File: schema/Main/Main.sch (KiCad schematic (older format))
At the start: 3 parts

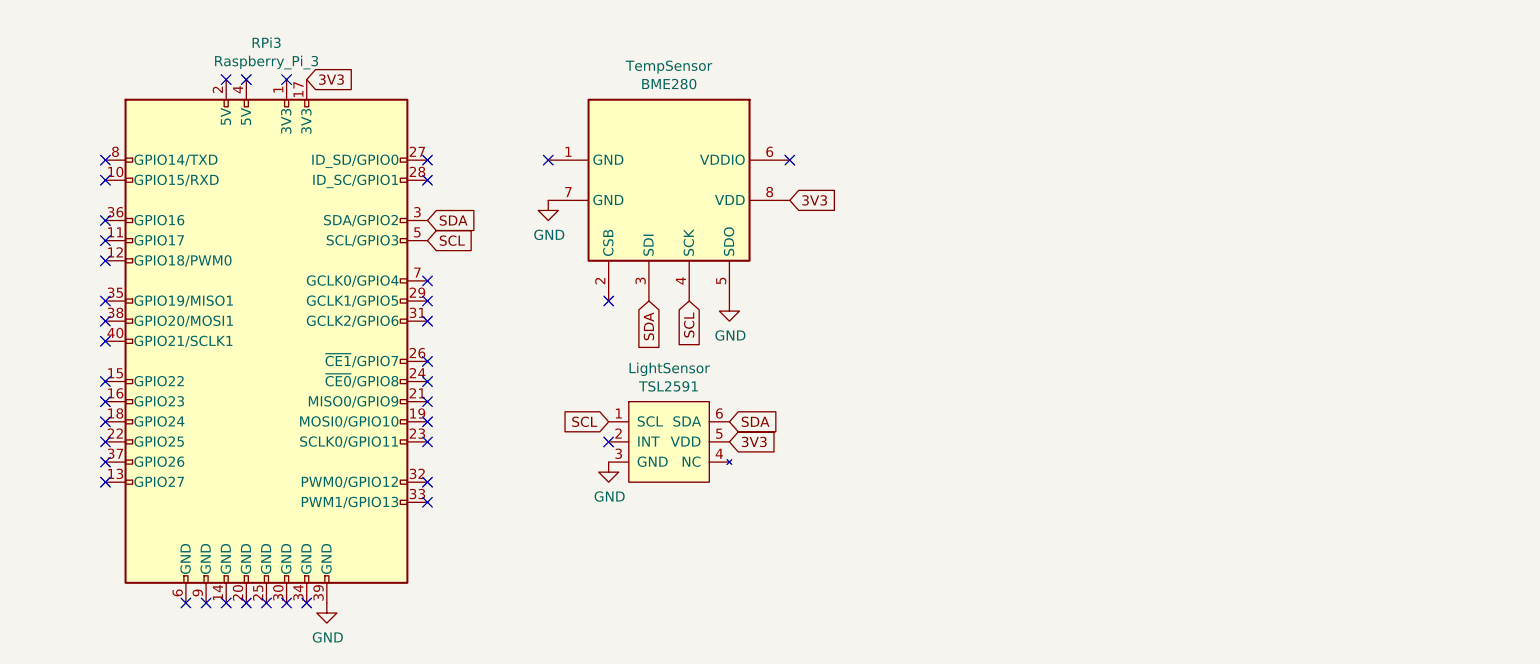
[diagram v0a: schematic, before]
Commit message: update
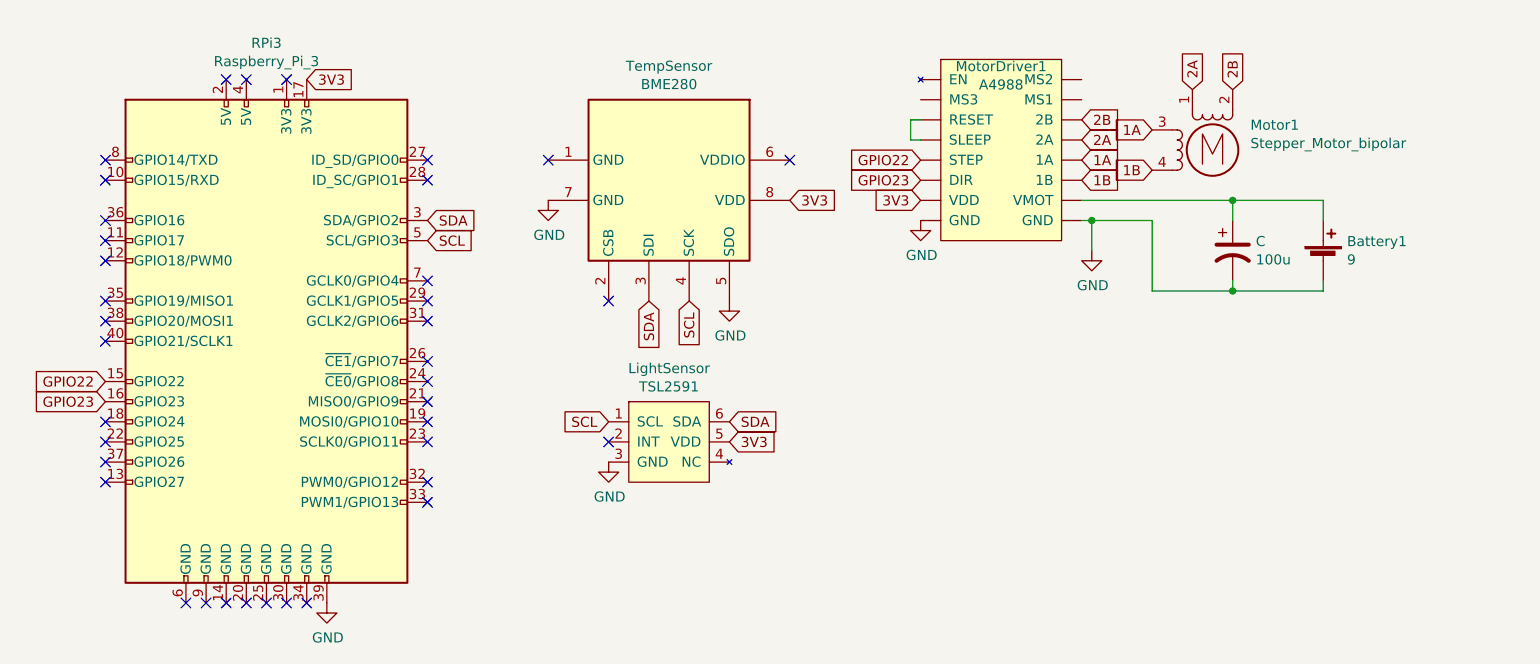
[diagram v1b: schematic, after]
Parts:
- added Battery1: 9, symbol Device:Battery_Cell
- added C: 100u, symbol Device:CP1
- added Motor1: Stepper_Motor_bipolar, symbol Motor:Stepper_Motor_bipolar
- added MotorDriver1: A4988, symbol A4998:A4988
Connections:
- net 3V3: now also MotorDriver1.~ (VMOT)
- net GND: now also Battery1.2 (-), C.2, MotorDriver1.~ (VMOT)
- net GPIO22: now reaches RPi3.15 (GPIO22)
- net GPIO22: now also MotorDriver1.~ (VMOT)
- net GPIO23: now reaches RPi3.16 (GPIO23)
- net GPIO23: now also MotorDriver1.~ (VMOT)
- new net: Battery1.1 (+), C.1, MotorDriver1.~ (VMOT)
- new net 1A: Motor1.3, MotorDriver1.~ (VMOT)
- new net 1B: Motor1.4, MotorDriver1.~ (VMOT)
- new net 2A: Motor1.1, MotorDriver1.~ (VMOT)
- new net 2B: Motor1.2 (-), MotorDriver1.~ (VMOT)
- no-connect marks 40 -> 38
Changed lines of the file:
@@
 NoConn ~ 900  2050
 NoConn ~ 900  2150
-NoConn ~ 900  2350
-NoConn ~ 900  2450
 NoConn ~ 900  2550
 NoConn ~ 900  2650
@@
 $EndComp
 NoConn ~ 3400 2650
+Wire Wire Line
+	4950 1150 4900 1150
+Wire Wire Line
+	4900 1150 4900 1050
+Wire Wire Line
+	4900 1050 4950 1050
+$Comp
+L Motor:Stepper_Motor_bipolar Motor1
+U 1 1 5E3C1483
+P 6400 1200
+F 0 "Motor1" H 6588 1324 50  0000 L CNN
+F 1 "Stepper_Motor_bipolar" H 6588 1233 50  0000 L CNN
+F 2 "" H 6410 1190 50  0001 C CNN
+F 3 "http://www.infineon.com/dgdl/Application-Note-TLE8110EE_driving_UniPolarStepperMotor_V1.1.pdf?fileId=db3a30431be39b97011be5d0aa0a00b0" H 6410 1190 50  0001 C CNN
+	1    6400 1200
+	1    0    0    -1
+$EndComp
+Text GLabel 4950 1450 0    50   Input ~ 0
+3V3
+$Comp
+L power:GND #PWR?
+U 1 1 5E3D2796
+P 4950 1550
+F 0 "#PWR?" H 4950 1300 50  0001 C CNN
+F 1 "GND" H 4955 1377 50  0000 C CNN
+F 2 "" H 4950 1550 50  0001 C CNN
+F 3 "" H 4950 1550 50  0001 C CNN
+	1    4950 1550
+	1    0    0    -1
+$EndComp
+$Comp
+L A4998:A4988 MotorDriver1
+U 1 1 5E3D5118
+P 5350 1850
+F 0 "MotorDriver1" H 5350 2915 50  0000 C CNN
+F 1 "A4988" H 5350 2824 50  0000 C CNN
+F 2 "" H 5350 2950 50  0001 C CNN
+F 3 "" H 5350 2950 50  0001 C CNN
+	1    5350 1850
+	1    0    0    -1
+$EndComp
+Text GLabel 900  2350 0    50   Input ~ 0
+GPIO22
+Text GLabel 900  2450 0    50   Input ~ 0
+GPIO23
+Text GLabel 4950 1250 0    50   Input ~ 0
+GPIO22
+Text GLabel 4950 1350 0    50   Input ~ 0
+GPIO23
+Text GLabel 5750 1350 2    50   Input ~ 0
+1B
+Text GLabel 6100 1300 0    50   Input ~ 0
+1B
+Text GLabel 5750 1250 2    50   Input ~ 0
+1A
+Text GLabel 5750 1150 2    50   Input ~ 0
+2A
+Text GLabel 5750 1050 2    50   Input ~ 0
+2B
+Text GLabel 6100 1100 0    50   Input ~ 0
+1A
+Text GLabel 6500 900  1    50   Input ~ 0
+2B
+Text GLabel 6300 900  1    50   Input ~ 0
+2A
+$Comp
+L Device:Battery_Cell Battery1
+U 1 1 5E3E99B9
+P 6950 1750
+F 0 "Battery1" H 7068 1846 50  0000 L CNN
+F 1 "9" H 7068 1755 50  0000 L CNN
+F 2 "" V 6950 1810 50  0001 C CNN
+F 3 "~" V 6950 1810 50  0001 C CNN
+	1    6950 1750
+	1    0    0    -1
+$EndComp
+$Comp
+L Device:CP1 C
+U 1 1 5E3ECAC5
+P 6500 1700
+F 0 "C" H 6615 1746 50  0000 L CNN
+F 1 "100u" H 6615 1655 50  0000 L CNN
+F 2 "" H 6500 1700 50  0001 C CNN
+F 3 "~" H 6500 1700 50  0001 C CNN
+	1    6500 1700
+	1    0    0    -1
+$EndComp
+Wire Wire Line
+	5750 1550 5800 1550
+Wire Wire Line
+	6100 1550 6100 1900
+Wire Wire Line
+	6950 1450 6950 1550
+Wire Wire Line
+	6950 1900 6950 1850
+Wire Wire Line
+	6100 1900 6500 1900
+Wire Wire Line
+	5750 1450 6500 1450
+Wire Wire Line
+	6500 1450 6500 1550
+Connection ~ 6500 1450
+Wire Wire Line
+	6500 1450 6950 1450
+Wire Wire Line
+	6500 1900 6500 1850
+Connection ~ 6500 1900
+Wire Wire Line
+	6500 1900 6950 1900
+$Comp
+L power:GND #PWR?
+U 1 1 5E4006C8
+P 5800 1700
+F 0 "#PWR?" H 5800 1450 50  0001 C CNN
+F 1 "GND" H 5805 1527 50  0000 C CNN
+F 2 "" H 5800 1700 50  0001 C CNN
+F 3 "" H 5800 1700 50  0001 C CNN
+	1    5800 1700
+	1    0    0    -1
+$EndComp
+Wire Wire Line
+	5800 1700 5800 1550
+Connection ~ 5800 1550
+Wire Wire Line
+	5800 1550 6100 1550
 $EndSCHEMATC

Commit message: MOTOR IS WORKING!!!!! mostly
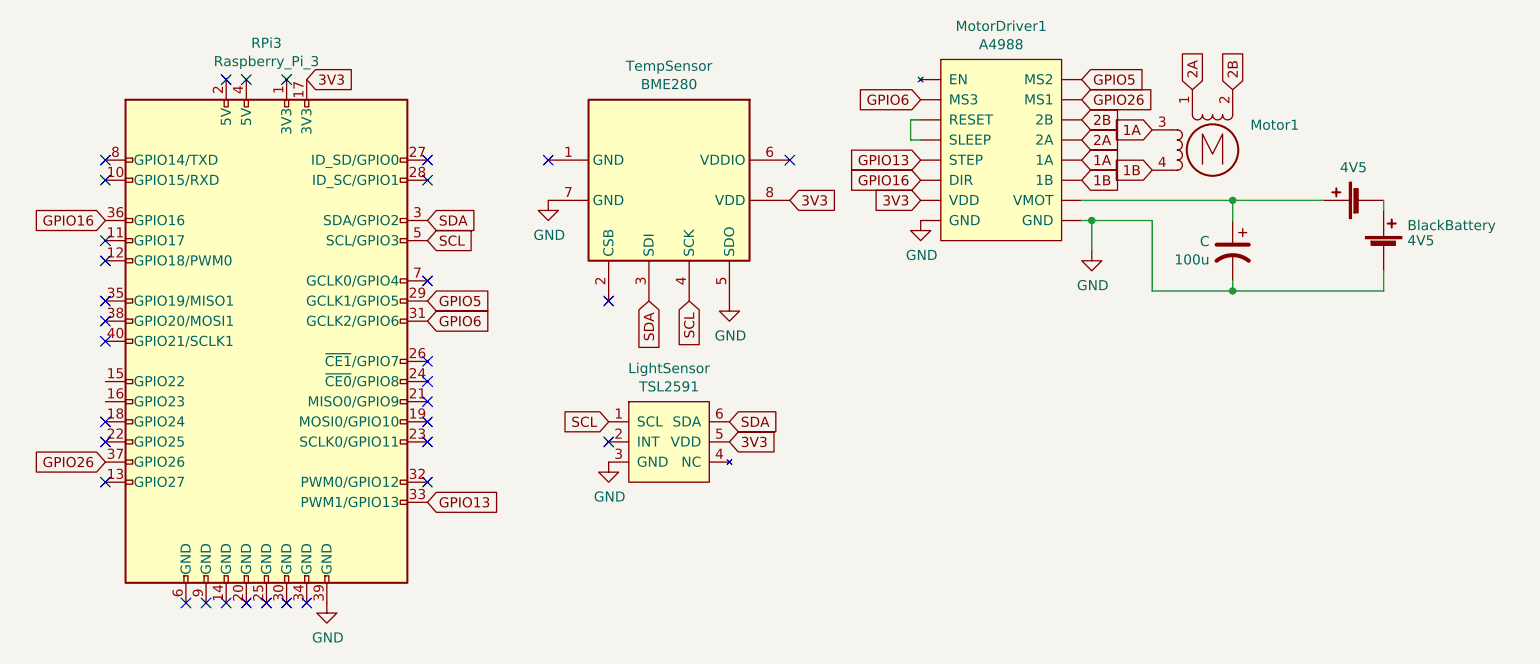
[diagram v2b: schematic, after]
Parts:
- removed Battery1: 9, symbol Device:Battery_Cell
- added Battery, BlackBattery: 4V5, symbol Device:Battery_Cell
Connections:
- net GND: now also BlackBattery.2 (-)
- net GPIO5: now reaches RPi3.29 (GCLK1/GPIO5)
- net GPIO5: now also MotorDriver1.~ (VMOT)
- net GPIO6: now reaches RPi3.31 (GCLK2/GPIO6)
- net GPIO6: now also MotorDriver1.~ (VMOT)
- net GPIO13: now reaches RPi3.33 (PWM1/GPIO13)
- net GPIO13: now also MotorDriver1.~ (VMOT)
- net GPIO16: now reaches RPi3.36 (GPIO16)
- net GPIO16: now also MotorDriver1.~ (VMOT)
- net GPIO26: now reaches RPi3.37 (GPIO26)
- net GPIO26: now also MotorDriver1.~ (VMOT)
- net at C.1, MotorDriver1.~ (VMOT): now also Battery.1 (+)
- net GPIO22: no longer names the net of RPi3.15 (GPIO22)
- net GPIO22: no longer MotorDriver1.~ (VMOT)
- net GPIO23: no longer names the net of RPi3.16 (GPIO23)
- net GPIO23: no longer MotorDriver1.~ (VMOT)
- new net: Battery.2 (-), BlackBattery.1 (+)
- no-connect marks 38 -> 33
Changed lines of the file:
@@
 NoConn ~ 900  1250
 NoConn ~ 900  1350
-NoConn ~ 900  1550
 NoConn ~ 900  1650
 NoConn ~ 900  1750
@@
 NoConn ~ 900  2550
 NoConn ~ 900  2650
-NoConn ~ 900  2750
 NoConn ~ 900  2850
 NoConn ~ 1300 3450
@@
 NoConn ~ 2500 1350
 NoConn ~ 2500 1850
-NoConn ~ 2500 1950
-NoConn ~ 2500 2050
 NoConn ~ 2500 2250
 NoConn ~ 2500 2350
@@
 NoConn ~ 2500 2650
 NoConn ~ 2500 2850
-NoConn ~ 2500 2950
 $Comp
 L power:GND #PWR?
@@
 P 6400 1200
 F 0 "Motor1" H 6588 1324 50  0000 L CNN
-F 1 "Stepper_Motor_bipolar" H 6588 1233 50  0000 L CNN
+F 1 "Stepper_Motor_bipolar" H 6588 1233 50  0001 L CNN
 F 2 "" H 6410 1190 50  0001 C CNN
 F 3 "http://www.infineon.com/dgdl/Application-Note-TLE8110EE_driving_UniPolarStepperMotor_V1.1.pdf?fileId=db3a30431be39b97011be5d0aa0a00b0" H 6410 1190 50  0001 C CNN
@@
 	1    0    0    -1
 $EndComp
-$Comp
-L A4998:A4988 MotorDriver1
-U 1 1 5E3D5118
-P 5350 1850
-F 0 "MotorDriver1" H 5350 2915 50  0000 C CNN
-F 1 "A4988" H 5350 2824 50  0000 C CNN
-F 2 "" H 5350 2950 50  0001 C CNN
-F 3 "" H 5350 2950 50  0001 C CNN
-	1    5350 1850
-	1    0    0    -1
-$EndComp
-Text GLabel 900  2350 0    50   Input ~ 0
-GPIO22
-Text GLabel 900  2450 0    50   Input ~ 0
-GPIO23
+Text GLabel 900  1550 0    50   Input ~ 0
+GPIO16
+Text GLabel 2500 2950 2    50   Input ~ 0
+GPIO13
+Text GLabel 4950 1350 0    50   Input ~ 0
+GPIO16
 Text GLabel 4950 1250 0    50   Input ~ 0
-GPIO22
-Text GLabel 4950 1350 0    50   Input ~ 0
-GPIO23
+GPIO13
 Text GLabel 5750 1350 2    50   Input ~ 0
 1B
@@
 2A
 $Comp
-L Device:Battery_Cell Battery1
-U 1 1 5E3E99B9
-P 6950 1750
-F 0 "Battery1" H 7068 1846 50  0000 L CNN
-F 1 "9" H 7068 1755 50  0000 L CNN
-F 2 "" V 6950 1810 50  0001 C CNN
-F 3 "~" V 6950 1810 50  0001 C CNN
-	1    6950 1750
-	1    0    0    -1
-$EndComp
-$Comp
 L Device:CP1 C
 U 1 1 5E3ECAC5
@@
 F 3 "~" H 6500 1700 50  0001 C CNN
 	1    6500 1700
-	1    0    0    -1
+	-1   0    0    -1
 $EndComp
 Wire Wire Line
@@
 Wire Wire Line
 	6100 1550 6100 1900
-Wire Wire Line
-	6950 1450 6950 1550
-Wire Wire Line
-	6950 1900 6950 1850
 Wire Wire Line
 	6100 1900 6500 1900
@@
 	6500 1900 6500 1850
 Connection ~ 6500 1900
-Wire Wire Line
-	6500 1900 6950 1900
 $Comp
 L power:GND #PWR?
@@
 Wire Wire Line
 	5800 1550 6100 1550
+$Comp
+L Device:Battery_Cell Battery
+U 1 1 5E5BAACC
+P 7150 1450
+F 0 "Battery" V 7405 1500 50  0001 C CNN
+F 1 "4V5" V 7313 1500 50  0000 C CNN
+F 2 "" V 7150 1510 50  0001 C CNN
+F 3 "~" V 7150 1510 50  0001 C CNN
+	1    7150 1450
+	0    -1   -1   0
+$EndComp
+Wire Wire Line
+	7250 1450 7250 1500
+Wire Wire Line
+	7250 1900 7250 1800
+Wire Wire Line
+	6500 1900 7250 1900
+$Comp
+L A4998:A4988 MotorDriver1
+U 1 1 5E5D37FE
+P 5350 1850
+F 0 "MotorDriver1" H 5350 3115 50  0000 C CNN
+F 1 "A4988" H 5350 3024 50  0000 C CNN
+F 2 "" H 5350 3150 50  0001 C CNN
+F 3 "" H 5350 3150 50  0001 C CNN
+	1    5350 1850
+	1    0    0    -1
+$EndComp
+Text GLabel 5750 950  2    50   Input ~ 0
+GPIO26
+Text GLabel 900  2750 0    50   Input ~ 0
+GPIO26
+Text GLabel 2500 1950 2    50   Input ~ 0
+GPIO5
+Text GLabel 2500 2050 2    50   Input ~ 0
+GPIO6
+Text GLabel 5750 850  2    50   Input ~ 0
+GPIO5
+Text GLabel 4950 950  0    50   Input ~ 0
+GPIO6
+$Comp
+L Device:Battery_Cell BlackBattery
+U 1 1 5E5BF867
+P 7250 1700
+F 0 "BlackBattery" H 7368 1796 50  0000 L BNN
+F 1 "4V5" H 7368 1750 50  0000 L CNN
+F 2 "" V 7250 1760 50  0001 C CNN
+F 3 "~" V 7250 1760 50  0001 C CNN
+	1    7250 1700
+	1    0    0    -1
+$EndComp
 $EndSCHEMATC
